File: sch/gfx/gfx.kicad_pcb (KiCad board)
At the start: 2 copper layers, 160 x 100 mm, 1623 parts, among them J1 DIN41612_B_3x32_Horizontal

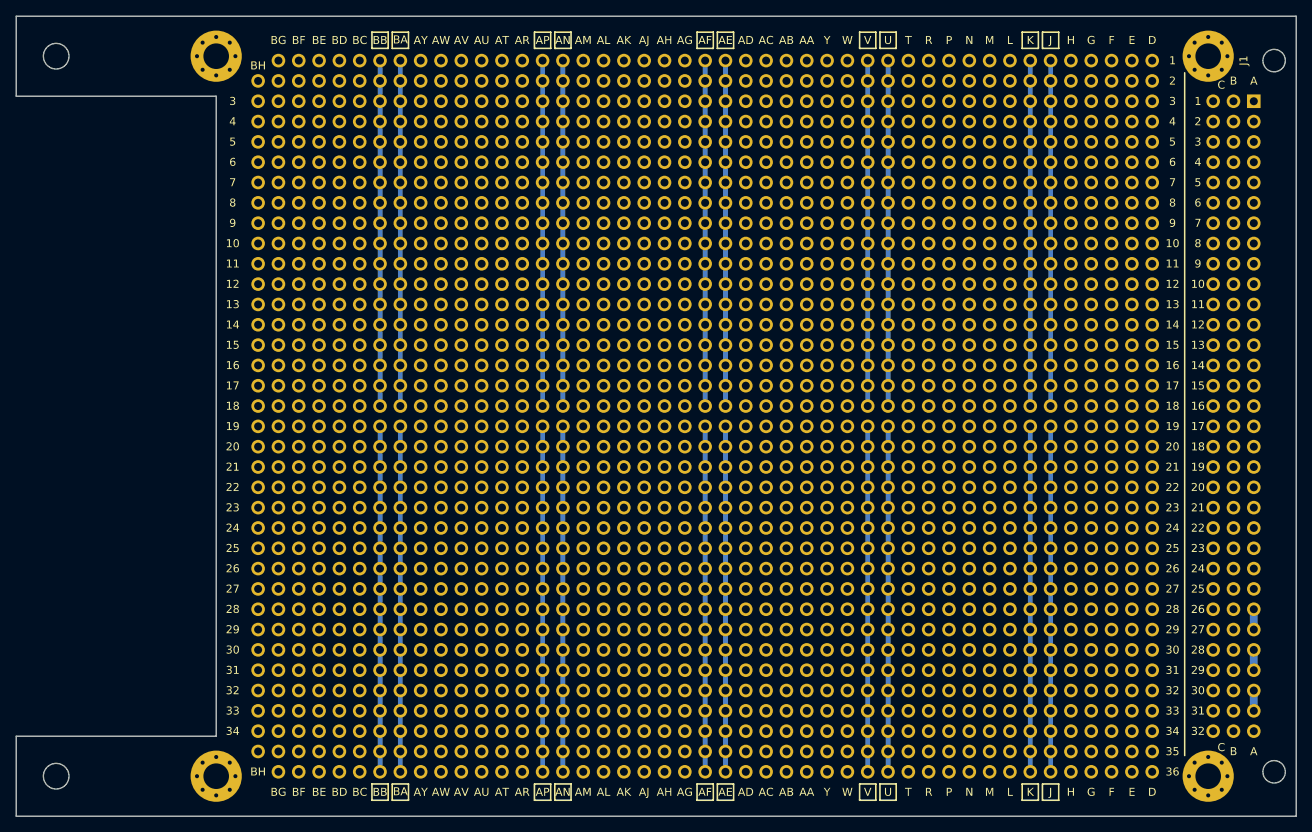
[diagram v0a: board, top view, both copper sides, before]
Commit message: gfx board, pcb version
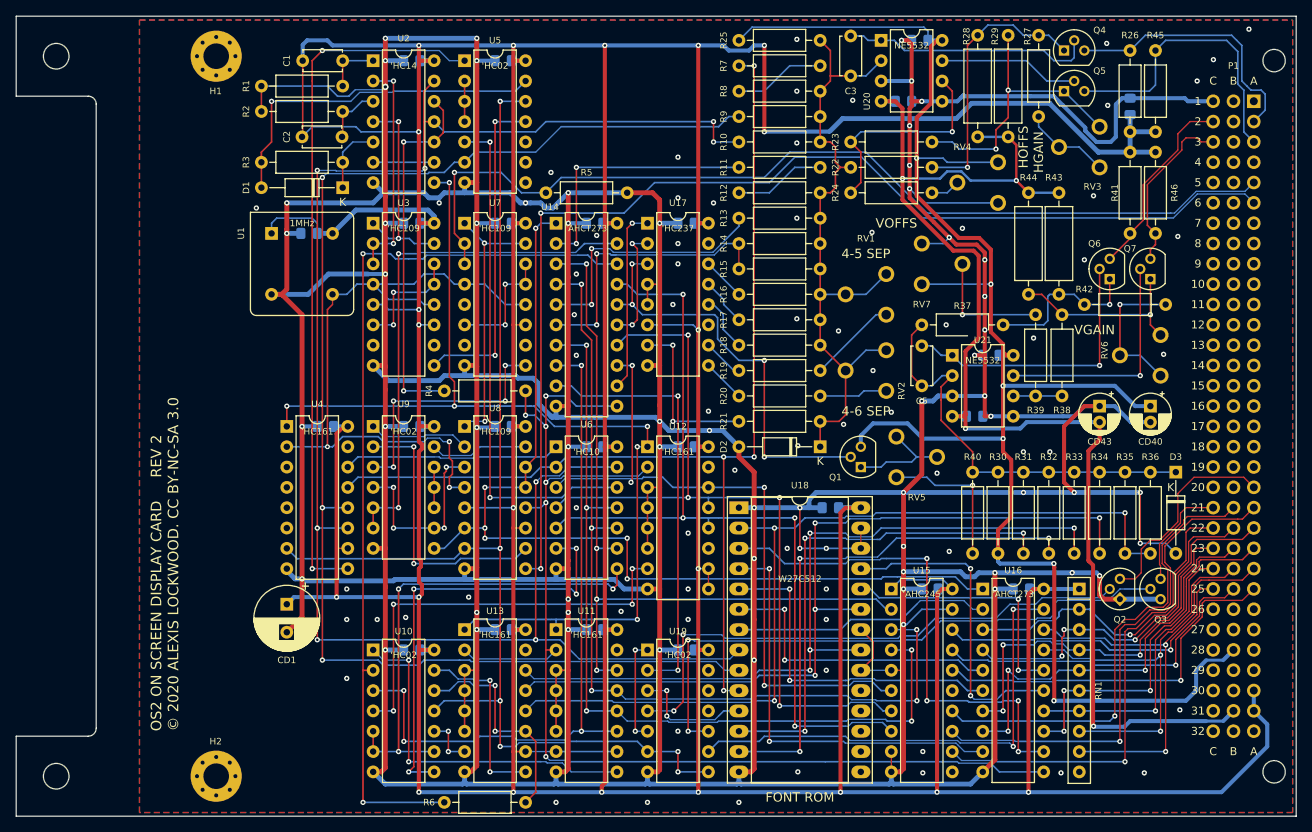
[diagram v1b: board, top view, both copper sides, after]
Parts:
- removed H4 (x2): MountingHole_3.2mm_M3_Pad_Via, MountingHole_3.2mm_M3_Pad_Via
- removed REF** (x1618): H, H
- added C1: 100p, Capacitor_THT:C_Disc_D4.7mm_W2.5mm_P5.00mm, F.Cu at (125.8, 35.6)
- added C2: 100p, Capacitor_THT:C_Disc_D4.7mm_W2.5mm_P5.00mm, F.Cu at (125.7, 45.1)
- added C3: 100p, Capacitor_THT:C_Disc_D4.7mm_W2.5mm_P5.00mm, F.Cu at (194.3, 37.5)
- added C5: 100p, Capacitor_THT:C_Disc_D4.7mm_W2.5mm_P5.00mm, F.Cu at (203.2, 76.2)
- added CD1: 470µ, Capacitor_THT:CP_Radial_D8.0mm_P3.50mm, F.Cu at (123.8, 103.5)
- added CD10: 1µ, Capacitor_SMD:C_0805_2012Metric_Pad1.15x1.40mm_HandSolder, B.Cu at (150.9, 81.3)
- added CD11: 1µ, Capacitor_SMD:C_0805_2012Metric_Pad1.15x1.40mm_HandSolder, B.Cu at (162.3, 55.9)
- added CD12: 1µ, Capacitor_SMD:C_0805_2012Metric_Pad1.15x1.40mm_HandSolder, B.Cu at (162.3, 83.8)
- added CD13: 1µ, Capacitor_SMD:C_0805_2012Metric_Pad1.15x1.40mm_HandSolder, B.Cu at (150.9, 106.7)
- added CD14: 1µ, Capacitor_SMD:C_0805_2012Metric_Pad1.15x1.40mm_HandSolder, B.Cu at (173.7, 55.9)
- added CD15: 1µ, Capacitor_SMD:C_0805_2012Metric_Pad1.15x1.40mm_HandSolder, B.Cu at (173.7, 83.8)
- added CD16: 1µ, Capacitor_SMD:C_0805_2012Metric_Pad1.15x1.40mm_HandSolder, B.Cu at (162.3, 106.7)
- added CD17: 1µ, Capacitor_SMD:C_0805_2012Metric_Pad1.15x1.40mm_HandSolder, B.Cu at (191.8, 91.4)
- added CD18: 1µ, Capacitor_SMD:C_0805_2012Metric_Pad1.15x1.40mm_HandSolder, B.Cu at (204.2, 101.6)
- added CD19: 1µ, Capacitor_SMD:C_0805_2012Metric_Pad1.15x1.40mm_HandSolder, B.Cu at (215.6, 101.6)
- added CD2: 1µ, Capacitor_SMD:C_0805_2012Metric_Pad1.15x1.40mm_HandSolder, B.Cu at (126.6, 57.1)
- added CD20: 1µ, Capacitor_SMD:C_0805_2012Metric_Pad1.15x1.40mm_HandSolder, B.Cu at (229.2, 41.3)
- added CD21: 1µ, Capacitor_SMD:C_0805_2012Metric_Pad1.15x1.40mm_HandSolder, B.Cu at (139.4, 109.2)
- added CD3: 1µ, Capacitor_SMD:C_0805_2012Metric_Pad1.15x1.40mm_HandSolder, B.Cu at (128.7, 81.3)
- added CD4: 1µ, Capacitor_SMD:C_0805_2012Metric_Pad1.15x1.40mm_HandSolder, B.Cu at (139.4, 35.6)
- added CD40: 47µ, Capacitor_THT:CP_Radial_D5.0mm_P2.00mm, F.Cu at (231.8, 78.7)
- added CD41: 1µ, Capacitor_SMD:C_0805_2012Metric_Pad1.15x1.40mm_HandSolder, B.Cu at (202.9, 33.0)
- added CD42: 1µ, Capacitor_SMD:C_0805_2012Metric_Pad1.15x1.40mm_HandSolder, B.Cu at (211.8, 72.4)
- added CD43: 47µ, Capacitor_THT:CP_Radial_D5.0mm_P2.00mm, F.Cu at (225.4, 78.7)
- added CD44: 1µ, Capacitor_SMD:C_0805_2012Metric_Pad1.15x1.40mm_HandSolder, B.Cu at (200.9, 40.6)
- added CD45: 1µ, Capacitor_SMD:C_0805_2012Metric_Pad1.15x1.40mm_HandSolder, B.Cu at (209.8, 80.0)
- added CD5: 1µ, Capacitor_SMD:C_0805_2012Metric_Pad1.15x1.40mm_HandSolder, B.Cu at (139.4, 55.9)
- added CD6: 1µ, Capacitor_SMD:C_0805_2012Metric_Pad1.15x1.40mm_HandSolder, B.Cu at (139.4, 81.3)
- added CD7: 1µ, Capacitor_SMD:C_0805_2012Metric_Pad1.15x1.40mm_HandSolder, B.Cu at (173.7, 109.2)
- added CD8: 1µ, Capacitor_SMD:C_0805_2012Metric_Pad1.15x1.40mm_HandSolder, B.Cu at (150.9, 35.6)
- added CD9: 1µ, Capacitor_SMD:C_0805_2012Metric_Pad1.15x1.40mm_HandSolder, B.Cu at (150.9, 55.9)
- added D1: 1N4148, Diode_THT:D_DO-35_SOD27_P10.16mm_Horizontal, F.Cu at (130.8, 51.4)
- added D2: 1N4148, Diode_THT:D_DO-35_SOD27_P10.16mm_Horizontal, F.Cu at (190.5, 83.8)
- added D3: 1N4148, Diode_THT:D_DO-35_SOD27_P10.16mm_Horizontal, F.Cu at (234.9, 87.0)
- added Q1: 2N3904, Package_TO_SOT_THT:TO-92, F.Cu at (195.6, 86.4)
- added Q2: 2N7000, Package_TO_SOT_THT:TO-92, F.Cu at (228.0, 102.9)
- added Q3: 2N7000, Package_TO_SOT_THT:TO-92, F.Cu at (233.0, 102.9)
- added Q4: 2N3904, Package_TO_SOT_THT:TO-92, F.Cu at (221.0, 34.3)
- added Q5: 2N3904, Package_TO_SOT_THT:TO-92, F.Cu at (221.0, 39.4)
- added Q6: 2N3904, Package_TO_SOT_THT:TO-92, F.Cu at (226.7, 62.9)
- added Q7: 2N3904, Package_TO_SOT_THT:TO-92, F.Cu at (231.8, 62.9)
- added R1: 82k, Resistor_THT:R_Axial_DIN0207_L6.3mm_D2.5mm_P10.16mm_Horizontal, F.Cu at (130.8, 38.7)
- added R10: 249k, Resistor_THT:R_Axial_DIN0207_L6.3mm_D2.5mm_P10.16mm_Horizontal, F.Cu at (190.5, 45.7)
- added R11: 68k, Resistor_THT:R_Axial_DIN0207_L6.3mm_D2.5mm_P10.16mm_Horizontal, F.Cu at (190.5, 48.9)
- added R12: 68k, Resistor_THT:R_Axial_DIN0207_L6.3mm_D2.5mm_P10.16mm_Horizontal, F.Cu at (190.5, 52.1)
- added R13: 68k, Resistor_THT:R_Axial_DIN0207_L6.3mm_D2.5mm_P10.16mm_Horizontal, F.Cu at (190.5, 55.2)
- added R14: 68k, Resistor_THT:R_Axial_DIN0207_L6.3mm_D2.5mm_P10.16mm_Horizontal, F.Cu at (190.5, 58.4)
- added R15: 68k, Resistor_THT:R_Axial_DIN0207_L6.3mm_D2.5mm_P10.16mm_Horizontal, F.Cu at (190.5, 61.6)
- added R16: 15k, Resistor_THT:R_Axial_DIN0207_L6.3mm_D2.5mm_P10.16mm_Horizontal, F.Cu at (190.5, 64.8)
- added R17: 7k5, Resistor_THT:R_Axial_DIN0207_L6.3mm_D2.5mm_P10.16mm_Horizontal, F.Cu at (190.5, 67.9)
- added R18: 4k99, Resistor_THT:R_Axial_DIN0207_L6.3mm_D2.5mm_P10.16mm_Horizontal, F.Cu at (190.5, 71.1)
- added R19: 18k, Resistor_THT:R_Axial_DIN0207_L6.3mm_D2.5mm_P10.16mm_Horizontal, F.Cu at (190.5, 74.3)
- added R2: 22k, Resistor_THT:R_Axial_DIN0207_L6.3mm_D2.5mm_P10.16mm_Horizontal, F.Cu at (130.8, 41.9)
- added R20: 8k2, Resistor_THT:R_Axial_DIN0207_L6.3mm_D2.5mm_P10.16mm_Horizontal, F.Cu at (190.5, 77.5)
- added R21: 4k99, Resistor_THT:R_Axial_DIN0207_L6.3mm_D2.5mm_P10.16mm_Horizontal, F.Cu at (190.5, 80.6)
- added R22: 1k6, Resistor_THT:R_Axial_DIN0207_L6.3mm_D2.5mm_P10.16mm_Horizontal, F.Cu at (194.3, 48.9)
- added R23: 1k6, Resistor_THT:R_Axial_DIN0207_L6.3mm_D2.5mm_P10.16mm_Horizontal, F.Cu at (204.5, 45.7)
- added R24: 7k5, Resistor_THT:R_Axial_DIN0207_L6.3mm_D2.5mm_P10.16mm_Horizontal, F.Cu at (194.3, 52.1)
- added R25: 6k2, Resistor_THT:R_Axial_DIN0207_L6.3mm_D2.5mm_P10.16mm_Horizontal, F.Cu at (190.5, 33.0)
- added R26: 75, Resistor_THT:R_Axial_DIN0207_L6.3mm_D2.5mm_P10.16mm_Horizontal, F.Cu at (229.2, 34.3)
- added R27: 100, Resistor_THT:R_Axial_DIN0207_L6.3mm_D2.5mm_P10.16mm_Horizontal, F.Cu at (217.8, 32.4)
- added R28: 1k, Resistor_THT:R_Axial_DIN0309_L9.0mm_D3.2mm_P12.70mm_Horizontal, F.Cu at (210.2, 45.1)
- added R29: 1k, Resistor_THT:R_Axial_DIN0309_L9.0mm_D3.2mm_P12.70mm_Horizontal, F.Cu at (214.0, 45.1)
- added R3: 10k, Resistor_THT:R_Axial_DIN0207_L6.3mm_D2.5mm_P10.16mm_Horizontal, F.Cu at (120.7, 48.3)
- added R30: 6k2, Resistor_THT:R_Axial_DIN0207_L6.3mm_D2.5mm_P10.16mm_Horizontal, F.Cu at (212.7, 87.0)
- added R31: 499k, Resistor_THT:R_Axial_DIN0207_L6.3mm_D2.5mm_P10.16mm_Horizontal, F.Cu at (215.9, 87.0)
- added R32: 249k, Resistor_THT:R_Axial_DIN0207_L6.3mm_D2.5mm_P10.16mm_Horizontal, F.Cu at (219.1, 87.0)
- added R33: 499k, Resistor_THT:R_Axial_DIN0207_L6.3mm_D2.5mm_P10.16mm_Horizontal, F.Cu at (222.2, 87.0)
- added R34: 249k, Resistor_THT:R_Axial_DIN0207_L6.3mm_D2.5mm_P10.16mm_Horizontal, F.Cu at (225.4, 87.0)
- added R35: 249k, Resistor_THT:R_Axial_DIN0207_L6.3mm_D2.5mm_P10.16mm_Horizontal, F.Cu at (228.6, 87.0)
- added R36: 249k, Resistor_THT:R_Axial_DIN0207_L6.3mm_D2.5mm_P10.16mm_Horizontal, F.Cu at (231.8, 87.0)
- added R37: 1k6, Resistor_THT:R_Axial_DIN0207_L6.3mm_D2.5mm_P10.16mm_Horizontal, F.Cu at (203.2, 68.6)
- added R38: 1k6, Resistor_THT:R_Axial_DIN0207_L6.3mm_D2.5mm_P10.16mm_Horizontal, F.Cu at (220.7, 67.3)
- added R39: 3k, Resistor_THT:R_Axial_DIN0207_L6.3mm_D2.5mm_P10.16mm_Horizontal, F.Cu at (217.4, 77.5)
- added R4: 10, Resistor_THT:R_Axial_DIN0207_L6.3mm_D2.5mm_P10.16mm_Horizontal, F.Cu at (143.5, 76.8)
- added R40: 820, Resistor_THT:R_Axial_DIN0207_L6.3mm_D2.5mm_P10.16mm_Horizontal, F.Cu at (209.6, 87.0)
- added R41: 75, Resistor_THT:R_Axial_DIN0207_L6.3mm_D2.5mm_P10.16mm_Horizontal, F.Cu at (229.2, 57.1)
- added R42: 100, Resistor_THT:R_Axial_DIN0207_L6.3mm_D2.5mm_P10.16mm_Horizontal, F.Cu at (223.5, 66.0)
- added R43: 1k, Resistor_THT:R_Axial_DIN0309_L9.0mm_D3.2mm_P12.70mm_Horizontal, F.Cu at (220.3, 52.1)
- added R44: 1k, Resistor_THT:R_Axial_DIN0309_L9.0mm_D3.2mm_P12.70mm_Horizontal, F.Cu at (216.5, 52.1)
- added R45: 75, Resistor_THT:R_Axial_DIN0207_L6.3mm_D2.5mm_P10.16mm_Horizontal, F.Cu at (232.4, 44.5)
- added R46: 75, Resistor_THT:R_Axial_DIN0207_L6.3mm_D2.5mm_P10.16mm_Horizontal, F.Cu at (232.4, 47.0)
- added R5: 6k8, Resistor_THT:R_Axial_DIN0207_L6.3mm_D2.5mm_P10.16mm_Horizontal, F.Cu at (166.4, 52.1)
- added R6: 3k3, Resistor_THT:R_Axial_DIN0207_L6.3mm_D2.5mm_P10.16mm_Horizontal, F.Cu at (143.5, 128.3)
- added R7: 499k, Resistor_THT:R_Axial_DIN0207_L6.3mm_D2.5mm_P10.16mm_Horizontal, F.Cu at (190.5, 36.2)
- added R8: 499k, Resistor_THT:R_Axial_DIN0207_L6.3mm_D2.5mm_P10.16mm_Horizontal, F.Cu at (190.5, 39.4)
- added R9: 499k, Resistor_THT:R_Axial_DIN0207_L6.3mm_D2.5mm_P10.16mm_Horizontal, F.Cu at (190.5, 42.5)
- added RN1: 1k, Resistor_THT:R_Array_SIP10, F.Cu at (222.9, 101.6)
- added RV1: 5k, alt-libs:stock_pot, F.Cu at (198.8, 67.3)
- added RV2: 5k, alt-libs:stock_pot, F.Cu at (198.8, 76.8)
- added RV3: 50, alt-libs:stock_pot, F.Cu at (225.4, 48.9)
- added RV4: 20k, alt-libs:stock_pot, F.Cu at (212.7, 53.3)
- added RV5: 10k, alt-libs:stock_pot, F.Cu at (200.0, 82.5)
- added RV6: 50, alt-libs:stock_pot, F.Cu at (233.0, 74.9)
- added RV7: 10k, alt-libs:stock_pot, F.Cu at (203.2, 58.4)
- added U1: 1MHz, Oscillator:Oscillator_DIP-8, F.Cu at (121.9, 57.1)
- added U10: 'HC02, Package_DIP:DIP-14_W7.62mm, F.Cu at (134.6, 109.2)
- added U11: 'HC161, Package_DIP:DIP-16_W7.62mm, F.Cu at (157.5, 106.7)
- added U12: 'HC161, Package_DIP:DIP-16_W7.62mm, F.Cu at (168.9, 83.8)
- added U13: 'HC161, Package_DIP:DIP-16_W7.62mm, F.Cu at (146.1, 106.7)
- added U14: 'AHCT273, Package_DIP:DIP-20_W7.62mm, F.Cu at (157.5, 55.9)
- added U15: 'AHC245, Package_DIP:DIP-20_W7.62mm, F.Cu at (199.4, 101.6)
- added U16: 'AHCT273, Package_DIP:DIP-20_W7.62mm, F.Cu at (210.8, 101.6)
- added U17: 'HC237, Package_DIP:DIP-16_W7.62mm, F.Cu at (168.9, 55.9)
- added U18: W27C512, Package_DIP:DIP-28_W15.24mm_Socket_LongPads, F.Cu at (180.3, 91.4)
- added U19: 'HC02, Package_DIP:DIP-14_W7.62mm, F.Cu at (168.9, 109.2)
- added U2: 'HC14, Package_DIP:DIP-14_W7.62mm, F.Cu at (134.6, 35.6)
- added U20: NE5532, Package_DIP:DIP-8_W7.62mm, F.Cu at (198.1, 33.0)
- added U21: NE5532, Package_DIP:DIP-8_W7.62mm, F.Cu at (207.0, 72.4)
- added U3: 'HC109, Package_DIP:DIP-16_W7.62mm, F.Cu at (134.6, 55.9)
- added U4: 'HC161, Package_DIP:DIP-16_W7.62mm, F.Cu at (123.8, 81.3)
- added U5: 'HC02, Package_DIP:DIP-14_W7.62mm, F.Cu at (146.1, 35.6)
- added U6: 'HC10, Package_DIP:DIP-14_W7.62mm, F.Cu at (157.5, 83.8)
- added U7: 'HC109, Package_DIP:DIP-16_W7.62mm, F.Cu at (146.1, 55.9)
- added U8: 'HC109, Package_DIP:DIP-16_W7.62mm, F.Cu at (146.1, 81.3)
- added U9: 'HC02, Package_DIP:DIP-14_W7.62mm, F.Cu at (134.6, 81.3)
- H1, H2: renamed from H4; value MountingHole_3.2mm_M3_Pad_Via -> HOLE; footprint MountingHole_3.2mm_M3_Pad_Via -> MountingHole:MountingHole_3.2mm_M3_Pad_Via
- P1: renamed from J1; value DIN41612_B_3x32_Horizontal -> DIN41612_M_3x32; footprint DIN41612_B_3x32_Horizontal -> alt-libs:DIN41612_B_3x32_Horizontal
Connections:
- H1 pad 1: gnd -> GND
- H2 pad 1: gnd -> GND
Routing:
- net GND: track 0.00 -> 1185.1 mm, vias 0 -> 130
- net VCC: track 0.00 -> 913.8 mm, vias 0 -> 21
- net /HDOT2: track 0.00 -> 215.4 mm, vias 0 -> 8
- net +15V: track 0.00 -> 213.8 mm, vias 0 -> 6
- net /HDOT1: track 0.00 -> 171.8 mm, vias 0 -> 3
- net -15V: track 0.00 -> 159.5 mm, vias 0 -> 4
- net RST#: track 0.00 -> 157.4 mm, vias 0 -> 6
- net POSCLK: track 0.00 -> 153.6 mm, vias 0 -> 6
- net RUN#: track 0.00 -> 149.7 mm, vias 0 -> 6
- net A6: track 0.00 -> 143.2 mm, vias 0 -> 2
- net /HDOT0: track 0.00 -> 134.3 mm, vias 0 -> 4
- net /PREDONE': track 0.00 -> 127.9 mm, vias 0 -> 2
- net RUN: track 0.00 -> 122.6 mm, vias 0 -> 6
- net /FLDREQ2: track 0.00 -> 121.1 mm, vias 0 -> 4
- net A5: track 0.00 -> 119.8 mm, vias 0 -> 1
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- added copper zone on B.Cu, net GND
- added copper zone on F.Cu, net GND
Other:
- outline, holes or cut-outs redrawn
- net class Default: clearance 0.2 -> 0.1778; trace_width 0.25 -> 0.1524; via_dia 0.8 -> 0.6096; via_drill 0.4 -> 0.3
- rule pad_to_mask_clearance: 0.05 -> 0
- rule trace_clearance: 0.2 -> 0.1778
- rule trace_min: 0.2 -> 0.1524
- rule via_min_size: 0.4 -> 0.6048
- board text added: "4-5 SEP"
- board text added: "4-6 SEP"
- board text added: "FONT ROM"
- board text added: "HGAIN"
- board text added: "HOFFS"
- board text added: "OS2 ON SCREEN DISPLAY CARD REV 2 © 2020 ALEXIS LOCKWOOD. CC BY-NC-SA 3.0"
- board text added: "VGAIN"
- board text added: "VOFFS"
- board text removed: "+10Vr"
- board text removed: "+12V"
- board text removed: "+15"
- board text removed: "+15V"
- board text removed: "+24V"
- board text removed: "+55V"
- board text removed: "+5V"
- board text removed: "+in1-"
- board text removed: "+in2-"
- board text removed: "+in3-"
- board text removed: "+in4-"
- board text removed: "+in5-"
- board text removed: "+sig-"
- board text removed: "+tsig-"
- board text removed: "-15"
- board text removed: "-15V"
- board text removed: "-55V"
- board text removed: "33"
- board text removed: "34"
- board text removed: "35"
- board text removed: "36"
- board text removed: "5V"
- board text removed: "AA"
- board text removed: "AB"
- board text removed: "AC"
- board text removed: "AD"
- board text removed: "AE"
- board text removed: "AF"
- board text removed: "AG"
- board text removed: "AH"
- board text removed: "AJ"
- board text removed: "AK"
- board text removed: "AL"
- board text removed: "AM"
- board text removed: "AN"
- board text removed: "AP"
- board text removed: "AR"
- board text removed: "AT"
- board text removed: "AU"
- board text removed: "AV"
- board text removed: "AW"
- board text removed: "AY"
- board text removed: "BA"
- board text removed: "BB"
- board text removed: "BC"
- board text removed: "BD"
- board text removed: "BE"
- board text removed: "BF"
- board text removed: "BG"
- board text removed: "BH"
- board text removed: "C0"
- board text removed: "C1"
- board text removed: "C2"
- board text removed: "C3"
- board text removed: "C4"
- board text removed: "C5"
- board text removed: "C6"
- board text removed: "CD1"
- board text removed: "CD40"
- board text removed: "CD43"
- board text removed: "CIN"
- board text removed: "D"
- board text removed: "D1"
- board text removed: "D2"
- board text removed: "D3"
- board text removed: "E"
- board text removed: "F"
- board text removed: "FS"
- board text removed: "G"
- board text removed: "GND"
- board text removed: "H"
- board text removed: "J"
- board text removed: "K"
- board text removed: "L"
- board text removed: "M"
- board text removed: "N"
- board text removed: "P"
- board text removed: "P0"
- board text removed: "P1"
- board text removed: "P2"
- board text removed: "Q1"
- board text removed: "Q2"
- board text removed: "Q3"
- board text removed: "Q4"
- board text removed: "Q5"
- board text removed: "Q6"
- board text removed: "Q7"
- board text removed: "R"
- board text removed: "R1"
- board text removed: "R10"
- board text removed: "R11"
- board text removed: "R12"
- board text removed: "R13"
- board text removed: "R14"
- board text removed: "R15"
- board text removed: "R16"
- board text removed: "R17"
- board text removed: "R18"
- board text removed: "R19"
- board text removed: "R2"
- board text removed: "R20"
- board text removed: "R21"
- board text removed: "R22"
- board text removed: "R23"
- board text removed: "R24"
- board text removed: "R25"
- board text removed: "R26"
- board text removed: "R27"
- board text removed: "R28"
- board text removed: "R29"
- board text removed: "R3"
- board text removed: "R30"
- board text removed: "R31"
- board text removed: "R32"
- board text removed: "R33"
- board text removed: "R34"
- board text removed: "R35"
- board text removed: "R36"
- board text removed: "R37"
- board text removed: "R39"
- board text removed: "R4"
- board text removed: "R40"
- board text removed: "R41"
- board text removed: "R42"
- board text removed: "R43"
- board text removed: "R44"
- board text removed: "R45"
- board text removed: "R46"
- board text removed: "R5"
- board text removed: "R6"
- board text removed: "R7"
- board text removed: "R8"
- board text removed: "R9"
- board text removed: "RN1"
- board text removed: "RV1"
- board text removed: "RV2"
- board text removed: "RV3"
- board text removed: "RV4"
- board text removed: "RV5"
- board text removed: "RV6"
- board text removed: "RV7"
- board text removed: "S"
- board text removed: "T"
- board text removed: "TIE IN AIR"
- board text removed: "U"
- board text removed: "U1"
- board text removed: "U10"
- board text removed: "U11"
- board text removed: "U12"
- board text removed: "U13"
- board text removed: "U14"
- board text removed: "U15"
- board text removed: "U16"
- board text removed: "U17"
- board text removed: "U18"
- board text removed: "U19"
- board text removed: "U2"
- board text removed: "U20"
- board text removed: "U21"
- board text removed: "U3"
- board text removed: "U4"
- board text removed: "U5"
- board text removed: "U6"
- board text removed: "U7"
- board text removed: "U8"
- board text removed: "U9"
- board text removed: "V"
- board text removed: "W"
- board text removed: "Y"
- board text removed: "a0"
- board text removed: "a1"
- board text removed: "a10"
- board text removed: "a11"
- board text removed: "a12"
- board text removed: "a13"
- board text removed: "a14"
- board text removed: "a15"
- board text removed: "a2"
- board text removed: "a3"
- board text removed: "a4"
- board text removed: "a5"
- board text removed: "a6"
- board text removed: "a7"
- board text removed: "a8"
- board text removed: "a9"
- board text removed: "s0"
- board text removed: "s1"
- board text removed: "s2"
- board text removed: "s3"
- board text removed: "s4"
- board text removed: "s5"
